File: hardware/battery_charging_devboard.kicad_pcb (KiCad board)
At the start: 2 copper layers, 119.5 x 87.5 mm, 127 parts, among them J1 Conn_01x02_Male, J2 USB_C_Receptacle_USB2.0, J3 DEBUG_CONN, J4 UART_CONN, J5 COMM_SELECT, J6 UART_SUPP, J7 OUT_SUP, Q1 DMP3036SSD, Q2 DMP3036SSD, Q3 MUN5335DW1T2G, SW1 BAT_IND, U1 RQ3E100BN, U10 L78L33_SO8, U2 RQ3E100BN, U3 BQ24725A, U4 RQ3E100BN, U5 RQ3E100BN, U6 RQ3E100BN, U7 CYPD3177, U8 T2N7002AK, U9 STM32F042F6Px

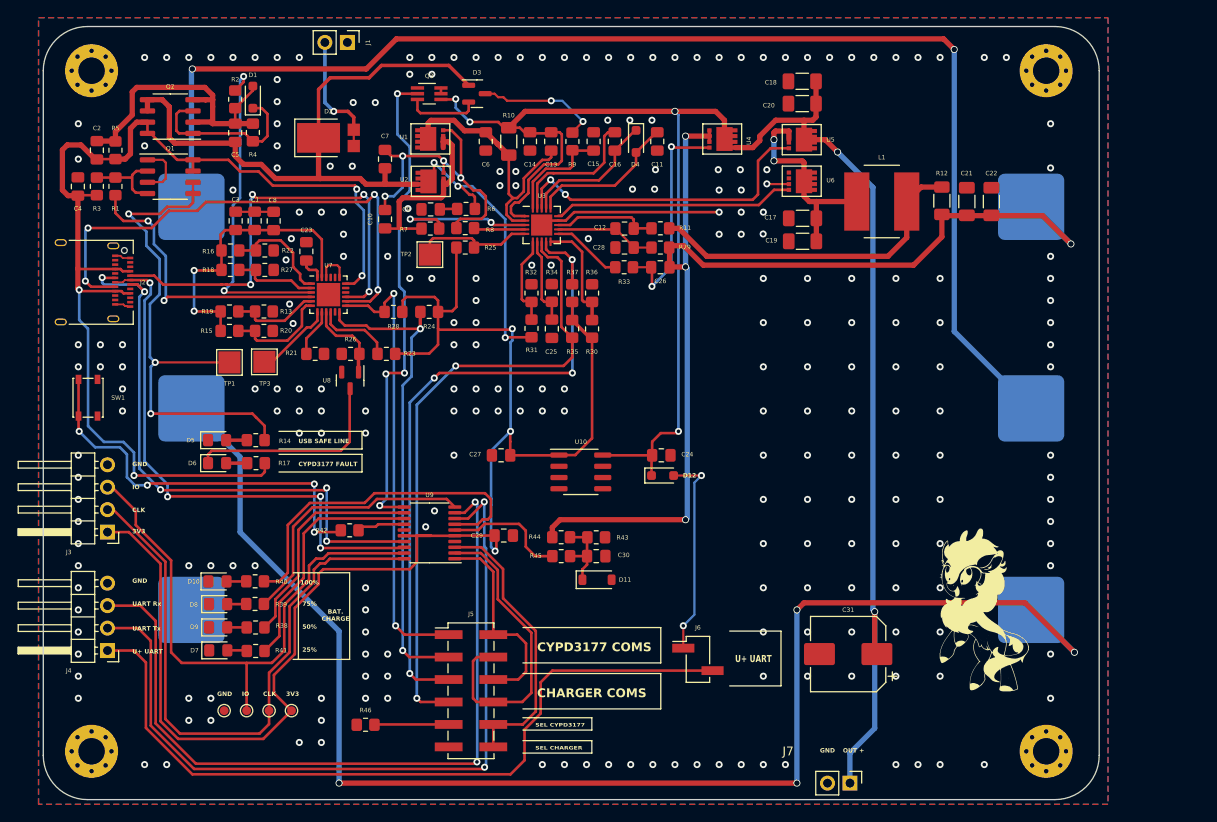
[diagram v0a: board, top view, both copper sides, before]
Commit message: Continuing routing
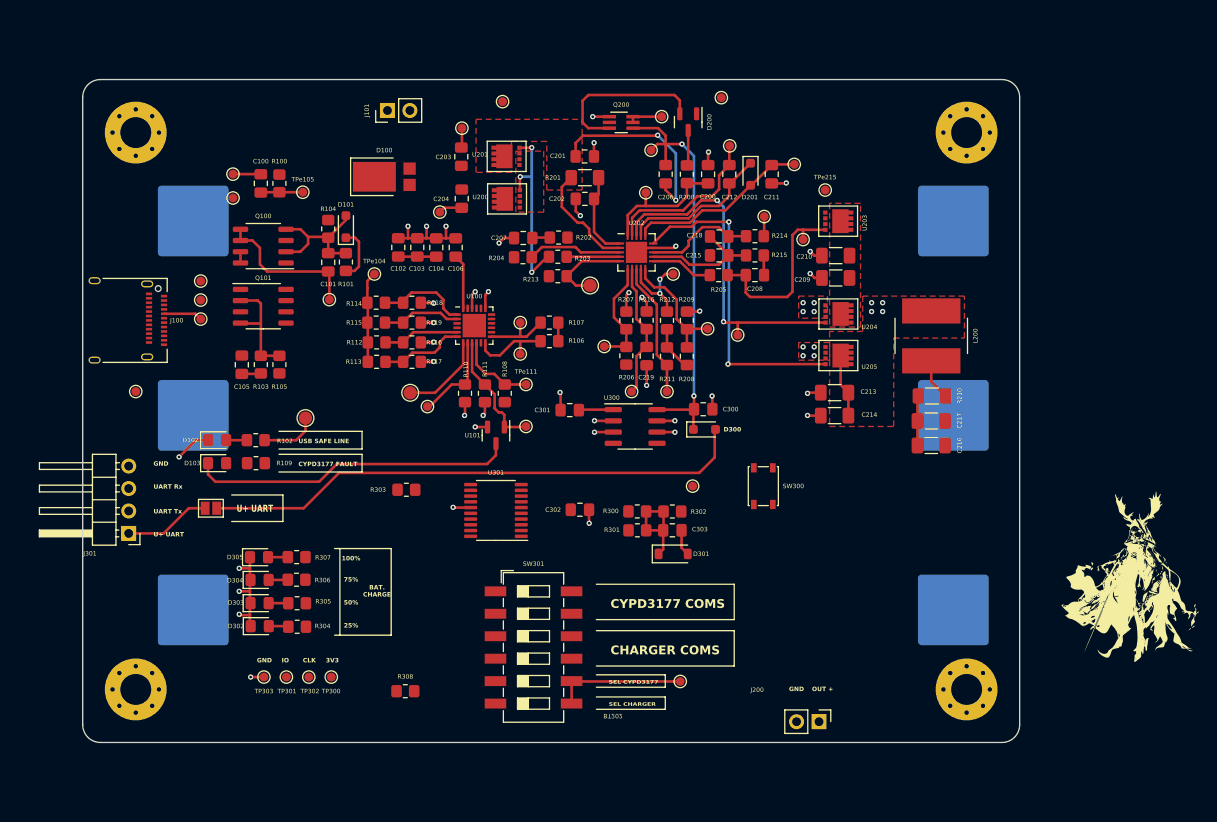
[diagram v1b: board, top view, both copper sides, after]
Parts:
- removed C31: 220u, Capacitor_SMD:CP_Elec_8x10
- removed J3: DEBUG_CONN, Connector_PinHeader_2.54mm:PinHeader_1x04_P2.54mm_Horizontal
- removed J5: COMM_SELECT, Connector_PinHeader_2.54mm:PinHeader_2x06_P2.54mm_Vertical_SMD
- removed REF** (x4): MountingHole_3mm_Pad_Via, MountingHole:MountingHole_3mm_Pad_Via
- added B501: MountingHole_Pad, MountingHole:MountingHole_3.5mm_Pad_Via, F.Cu at (49.0, 51.0)
- added B502: MountingHole_Pad, MountingHole:MountingHole_3.5mm_Pad_Via, F.Cu at (49.0, 114.0)
- added B503: MountingHole_Pad, MountingHole:MountingHole_3.5mm_Pad_Via, F.Cu at (143.0, 51.0)
- added B504: MountingHole_Pad, MountingHole:MountingHole_3.5mm_Pad_Via, F.Cu at (143.0, 114.0)
- added SW301: SW_DIP_x06, Button_Switch_SMD:SW_DIP_SPSTx06_Slide_6.7x16.8mm_W8.61mm_P2.54mm_LowProfile, F.Cu at (94.0, 109.2)
- added TPe100: TestPoint, TestPoint:TestPoint_Pad_D1.0mm, F.Cu at (60.0, 58.4)
- added TPe101: TestPoint, TestPoint:TestPoint_Pad_D1.0mm, F.Cu at (60.0, 55.7)
- added TPe102: TestPoint, TestPoint:TestPoint_Pad_D1.0mm, F.Cu at (56.4, 67.8)
- added TPe103: TestPoint, TestPoint:TestPoint_Pad_D1.0mm, F.Cu at (56.4, 70.0)
- added TPe104: TestPoint, TestPoint:TestPoint_Pad_D1.0mm, F.Cu at (76.0, 67.0)
- added TPe105: TestPoint, TestPoint:TestPoint_Pad_D1.0mm, F.Cu at (67.9, 57.8)
- added TPe106: TestPoint, TestPoint:TestPoint_Pad_D1.0mm, F.Cu at (70.9, 69.9)
- added TPe107: TestPoint, TestPoint:TestPoint_Pad_D1.0mm, F.Cu at (92.5, 72.5)
- added TPe108: TestPoint, TestPoint:TestPoint_Pad_D1.0mm, F.Cu at (56.4, 72.1)
- added TPe109: TestPoint, TestPoint:TestPoint_Pad_D1.0mm, F.Cu at (49.0, 80.3)
- added TPe110: TestPoint, TestPoint:TestPoint_Pad_D1.0mm, F.Cu at (92.5, 76.0)
- added TPe111: TestPoint, TestPoint:TestPoint_Pad_D1.0mm, F.Cu at (93.2, 79.5)
- added TPe112: TestPoint, TestPoint:TestPoint_Pad_D1.0mm, F.Cu at (82.0, 82.0)
- added TPe113: TestPoint, TestPoint:TestPoint_Pad_D1.0mm, F.Cu at (93.2, 84.2)
- added TPe200: TestPoint, TestPoint:TestPoint_Pad_D1.0mm, F.Cu at (115.2, 47.0)
- added TPe201: TestPoint, TestPoint:TestPoint_Pad_D1.0mm, F.Cu at (108.5, 49.2)
- added TPe202: TestPoint, TestPoint:TestPoint_Pad_D1.0mm, F.Cu at (106.7, 57.8)
- added TPe203: TestPoint, TestPoint:TestPoint_Pad_D1.0mm, F.Cu at (83.4, 60.0)
- added TPe204: TestPoint, TestPoint:TestPoint_Pad_D1.0mm, F.Cu at (107.3, 53.0)
- added TPe206: TestPoint, TestPoint:TestPoint_Pad_D1.0mm, F.Cu at (85.9, 50.5)
- added TPe207: TestPoint, TestPoint:TestPoint_Pad_D1.0mm, F.Cu at (124.5, 63.1)
- added TPe208: TestPoint, TestPoint:TestPoint_Pad_D1.0mm, F.Cu at (90.5, 47.5)
- added TPe209: TestPoint, TestPoint:TestPoint_Pad_D1.0mm, F.Cu at (123.5, 54.6)
- added TPe210: TestPoint, TestPoint:TestPoint_Pad_D1.0mm, F.Cu at (102.0, 75.2)
- added TPe211: TestPoint, TestPoint:TestPoint_Pad_D1.0mm, F.Cu at (113.7, 73.2)
- added TPe212: TestPoint, TestPoint:TestPoint_Pad_D1.0mm, F.Cu at (117.1, 73.9)
- added TPe213: TestPoint, TestPoint:TestPoint_Pad_D1.0mm, F.Cu at (120.1, 60.5)
- added TPe214: TestPoint, TestPoint:TestPoint_Pad_D1.0mm, F.Cu at (116.2, 52.5)
- added TPe215: TestPoint, TestPoint:TestPoint_Pad_D1.0mm, F.Cu at (127.0, 57.5)
- added TPe216: TestPoint, TestPoint:TestPoint_Pad_D1.0mm, F.Cu at (109.1, 80.3)
- added TPe217: TestPoint, TestPoint:TestPoint_Pad_D1.0mm, F.Cu at (109.8, 67.0)
- added TPe218: TestPoint, TestPoint:TestPoint_Pad_D1.0mm, F.Cu at (105.1, 80.3)
- added TPe300: TestPoint, TestPoint:TestPoint_Pad_D1.0mm, F.Cu at (112.0, 91.0)
- added TPe301: TestPoint, TestPoint:TestPoint_Pad_D1.0mm, F.Cu at (110.6, 113.1)
- J300: renamed from J6; footprint Connector_PinHeader_2.54mm:PinHeader_1x02_P2.54mm_Vertical_SMD_Pin1Left -> Jumper:SolderJumper-2_P1.3mm_Open_Pad1.0x1.5mm
- TP100: renamed from TP1; footprint TestPoint:TestPoint_Pad_2.5x2.5mm -> TestPoint:TestPoint_Pad_D1.5mm
- TP101: renamed from TP3; footprint TestPoint:TestPoint_Pad_2.5x2.5mm -> TestPoint:TestPoint_Pad_D1.5mm
- TP200: renamed from TP2; footprint TestPoint:TestPoint_Pad_2.5x2.5mm -> TestPoint:TestPoint_Pad_D1.5mm
- moved SW300 77.1 mm to (120.0, 91.0)
- moved J300 57.7 mm to (57.5, 93.5), turned to 180 degrees
- moved C216 28.4 mm to (139.0, 86.4), turned to 180 degrees
- moved C105 27.4 mm to (61.0, 77.3)
- moved R103 27.4 mm to (63.1, 77.2)
- moved R105 27.4 mm to (65.2, 77.2)
- moved C217 25.1 mm to (139.0, 83.6), turned to 180 degrees
- moved D200 24.1 mm to (111.5, 49.8), turned to -90 degrees
- moved R210 22.1 mm to (139.1, 80.8), turned to 0 degrees
- moved Q200 22.0 mm to (103.9, 49.9)
- moved U204 20.2 mm to (128.5, 71.5)
- moved U205 20.2 mm to (128.5, 76.2)
- moved C209 20.1 mm to (128.2, 67.4)
- moved C210 20.1 mm to (128.2, 64.9)
- moved C213 20.1 mm to (128.1, 80.4)
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- renumbered BT1 to BT200, BT2 to BT201, BT3 to BT202, C2 to C100, C5 to C101, C3 to C102, C1 to C103, C8 to C104, C4 to C105, C23 to C106, C15 to C200, C6 to C201, C14 to C202, C7 to C203, C10 to C204, C13 to C206, C9 to C207, C26 to C208, C20 to C209, C18 to C210, C11 to C211, C16 to C212, C17 to C213, C19 to C214, C28 to C215, C22 to C216, C21 to C217, C12 to C218, C25 to C219, C24 to C300, C27 to C301, C29 to C302, C30 to C303, D2 to D100, D1 to D101, D5 to D102, D6 to D103, D3 to D200, D4 to D201, D12 to D300, D11 to D301, D7 to D302, D9 to D303, D8 to D304, D10 to D305, J2 to J100, J1 to J101, J7 to J200, J4 to J301, L1 to L200, Q2 to Q100, Q1 to Q101, Q3 to Q200, R5 to R100, R4 to R101, R14 to R102, R3 to R103, R2 to R104, R1 to R105, R24 to R106, R28 to R107, R23 to R108, R17 to R109, R21 to R110, R26 to R111, R19 to R112, R15 to R113, R16 to R114, R18 to R115, R13 to R116, R20 to R117, R22 to R118, R27 to R119, R9 to R200, R10 to R201, R6 to R202, R8 to R203, R7 to R204, R33 to R205, R31 to R206, R32 to R207, R30 to R208, R36 to R209, R12 to R210, R35 to R211, R37 to R212, R25 to R213, R11 to R214, R29 to R215, R34 to R216, R44 to R300, R45 to R301, R43 to R302, R42 to R303, R41 to R304, R38 to R305, R39 to R306, R40 to R307, R46 to R308, SW1 to SW300, TP6 to TP300, TP5 to TP301, TP7 to TP302, TP4 to TP303, U7 to U100, U8 to U101, U2 to U200, U1 to U201, U3 to U202, U4 to U203, U5 to U204, U6 to U205, U10 to U300, U9 to U301
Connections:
- C212 pad 1: Net-(U3-PHASE) -> Net-(U202-PHASE)
- C213 pad 2: Net-(C17-Pad2) -> Net-(U202-PHASE)
- C214 pad 2: Net-(C17-Pad2) -> Net-(U202-PHASE)
- L200 pad 1: Net-(C17-Pad2) -> Net-(U202-PHASE)
- U100 pad 11: unconnected-(U7-VDC_OUT-Pad11) -> V_USB_OUT
- U202 pad 19: Net-(U3-PHASE) -> Net-(U202-PHASE)
- U204 pad 1: Net-(C17-Pad2) -> Net-(U202-PHASE)
- U204 pad 2: Net-(C17-Pad2) -> Net-(U202-PHASE)
- U204 pad 3: Net-(C17-Pad2) -> Net-(U202-PHASE)
- U205 pad 5: Net-(C17-Pad2) -> Net-(U202-PHASE)
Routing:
- net VREG_3V3: track 177.3 -> 11.1 mm, vias 3 -> 0
- net Net-(BT201--): track 161.7 -> 0.00 mm, vias 4 -> 0
- net POWER_SYSTEM: track 207.1 -> 58.1 mm, vias 6 -> 2
- net Net-(BT200--): track 148.0 -> 0.00 mm, vias 2 -> 0
- net USB_C_BUS: track 127.0 -> 8.21 mm, vias 4 -> 0
- net uC_adc_battery: track 124.1 -> 7.89 mm, vias 4 -> 0
- net /microcontroller/uC_uart_tx: track 89.3 -> 0.00 mm, vias 2 -> 0
- net /microcontroller/uC_uart_rx: track 88.4 -> 0.00 mm, vias 2 -> 0
- net V_USB_OUT: track 102.1 -> 17.0 mm, vias 3 -> 0
- net Net-(J300-Pin_2): track 87.5 -> 9.83 mm
- net /microcontroller/uc_swclk: track 69.9 -> 0.00 mm
- net USB_C_D-: track 67.0 -> 0.00 mm, vias 5 -> 0
- net I2C_CLK_CHRG: track 75.0 -> 9.91 mm, vias 4 -> 2
- net /microcontroller/uC_swdio: track 63.3 -> 0.00 mm
- net USB_C_D+: track 62.4 -> 0.00 mm, vias 4 -> 0
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- added copper zone on In1.Cu, net GND
- added copper zone on F.Cu, net Net-(C204-Pad1)
- added copper zone on F.Cu, net Net-(U202-ACP)
- added copper zone on F.Cu, net Net-(U202-PHASE)
- added copper zone on In2.Cu, net Net-(U202-PHASE)
- added copper zone on F.Cu, net POWER_SYSTEM
- removed copper zone on B.Cu, net GND
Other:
- board size 119.5 x 87.5 mm -> 106 x 75 mm
- copper layers 2 -> 4
